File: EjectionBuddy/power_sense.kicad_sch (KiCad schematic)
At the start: 7 parts, among them U2 INA199B2

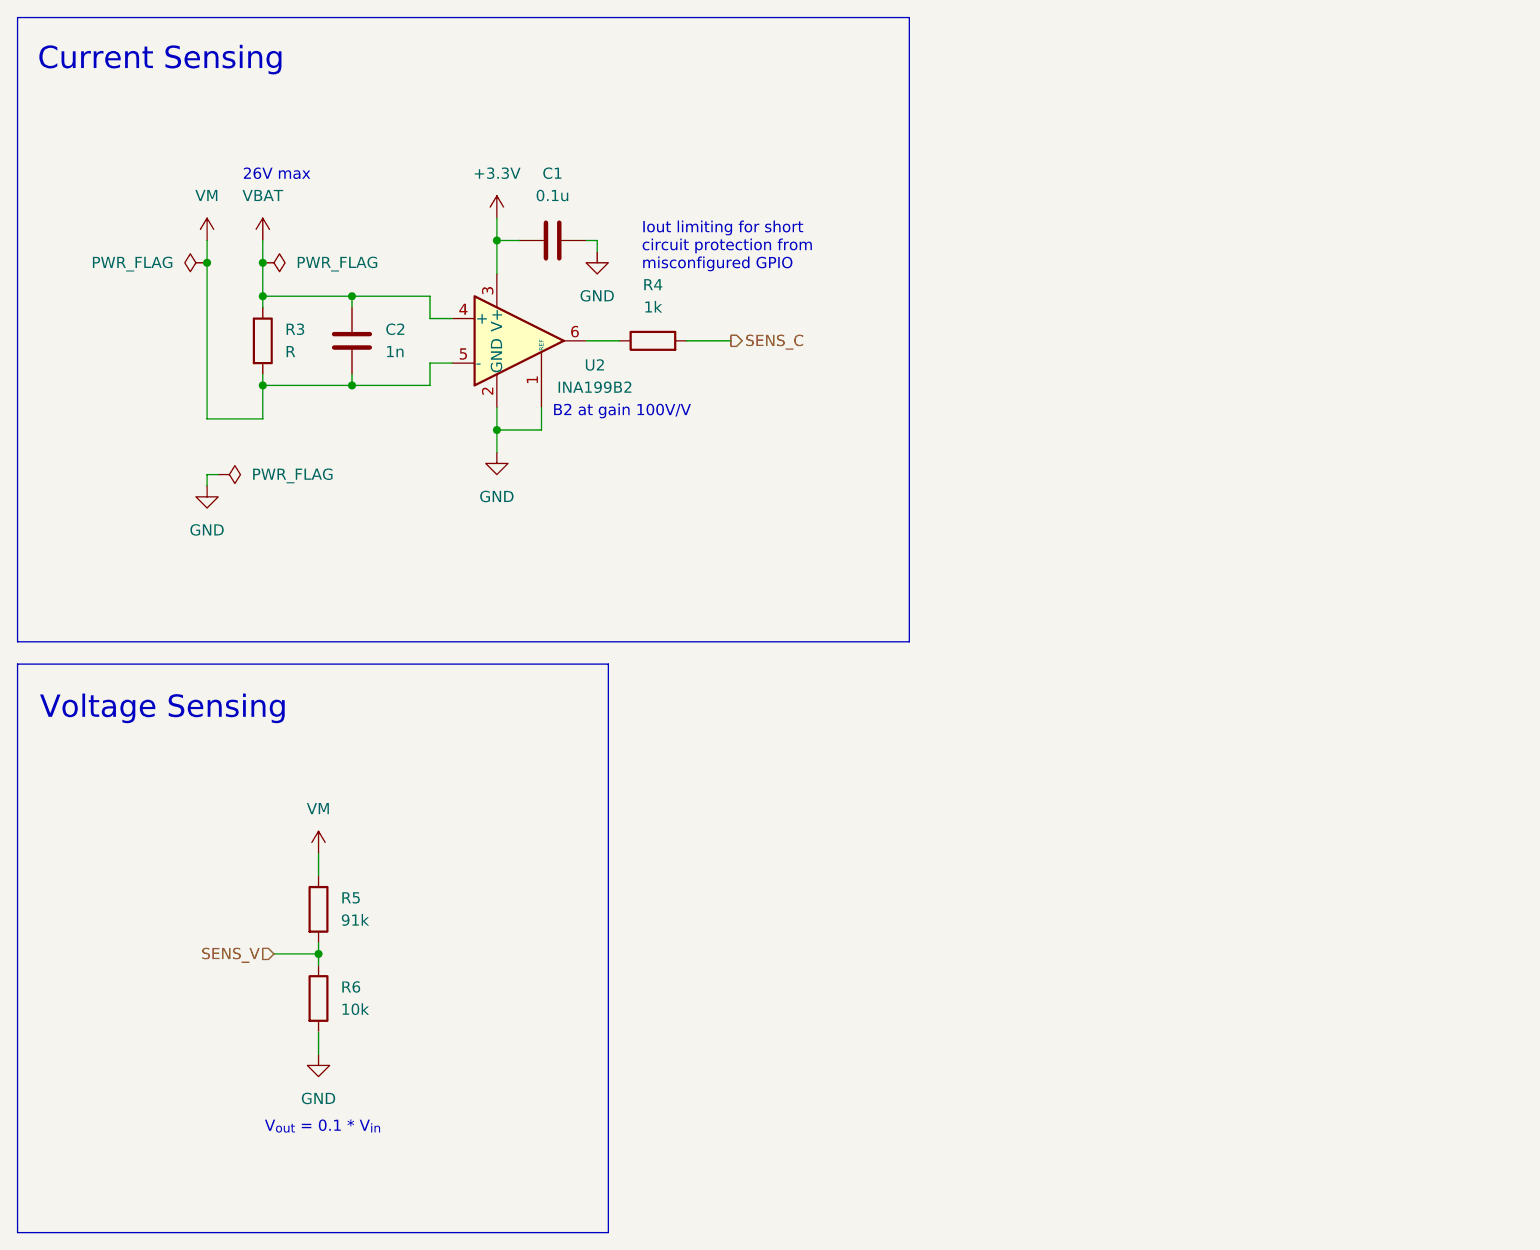
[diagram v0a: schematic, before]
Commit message: Finished! QR and instruction pending
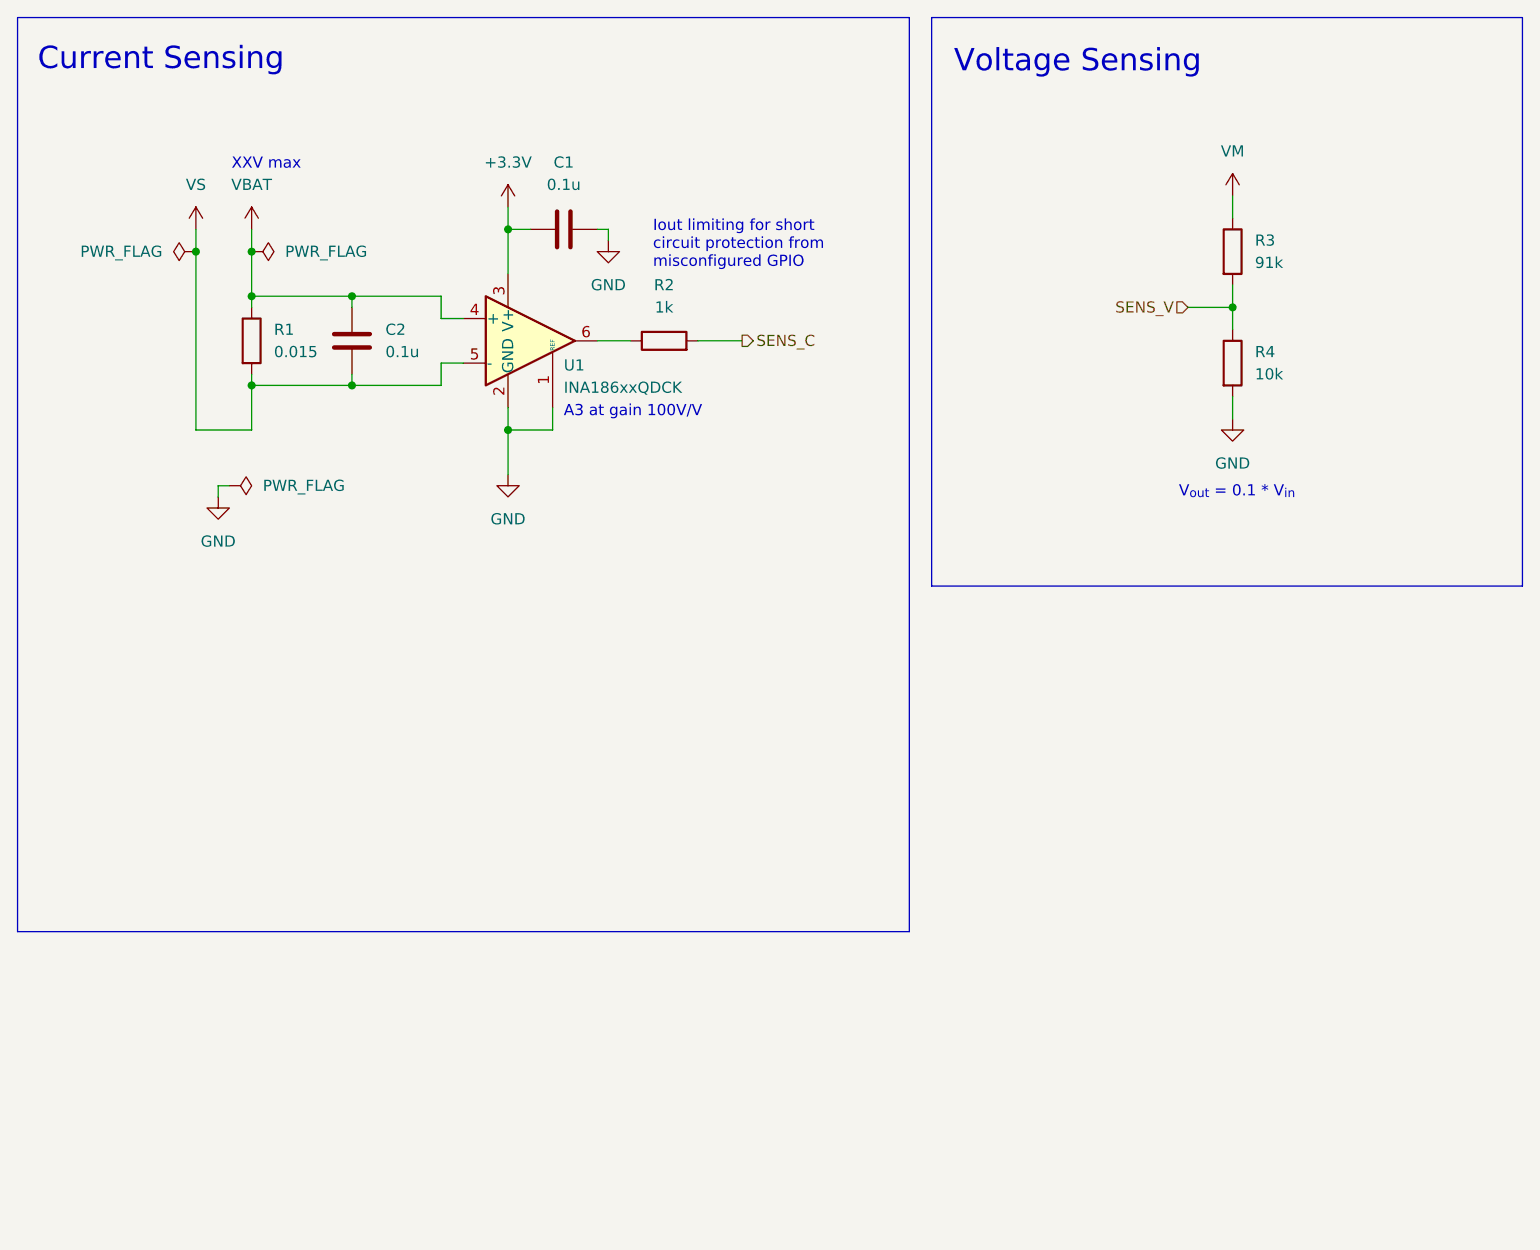
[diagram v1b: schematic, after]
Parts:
- removed U2: INA199B2, Package_TO_SOT_SMD:SOT-363_SC-70-6, symbol Amplifier_Current:INA199xxDCK
- added U1: INA186xxQDCK, Package_TO_SOT_SMD:SOT-363_SC-70-6, symbol INA186:INA186xxQDCK
- C2: value 1n -> 0.1u
- R1: renamed from R3; value R -> 0.015; footprint FirstAero:ESC_CurrentSense_R_2x1206 -> Resistor_SMD:R_0805_2012Metric
- renumbered R4 to R2, R5 to R3, R6 to R4
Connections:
- net +3.3V: now also U1.3 (V+)
- net GND: now also U1.1 (REF), U1.2 (GND)
- net VBAT: now also U1.4 (+)
- net VM: no longer C2.2, R1.2
- net at R2.1: now also U1.6
- new net VS: C2.2, R1.2, U1.5 (-)
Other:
- note added: "A3 at gain 100V/V"
- note added: "XXV max"
- note removed: "26V max"
- note removed: "B2 at gain 100V/V"
- moved on the sheet: C1, R1, R2, R3, R4
